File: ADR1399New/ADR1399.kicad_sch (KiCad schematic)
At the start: 95 parts, among them J1 GNDF_SPARE, J10 Conn_01x01_Male, J11 Conn_01x01, J2 10V, J3 PT100, J4 Guards, J5 7V, J6 Conn_01x02_Male, J7 Conn_01x02_Male, J8 Conn_01x02_Male, J9 Conn_01x02_Male, Q1 BC817, U1 OPA2182xD, U2 OPA2209xD, U3 OPA2182xD, U4 LM399, U5 LM7905_TO220, U6 LM7815_TO220, U7 LM7805_TO220, U8 OPA2182xD

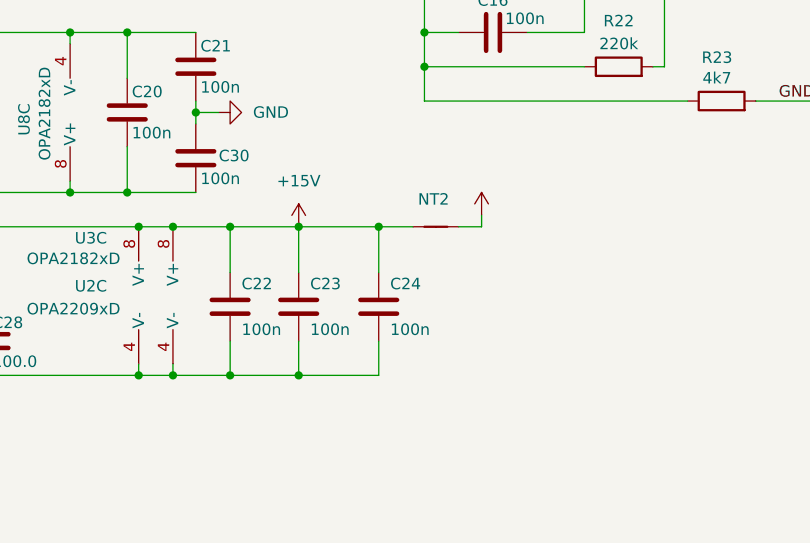
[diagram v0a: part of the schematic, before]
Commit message: Update KiCad project and backup files- just before format R9 7900x SSD
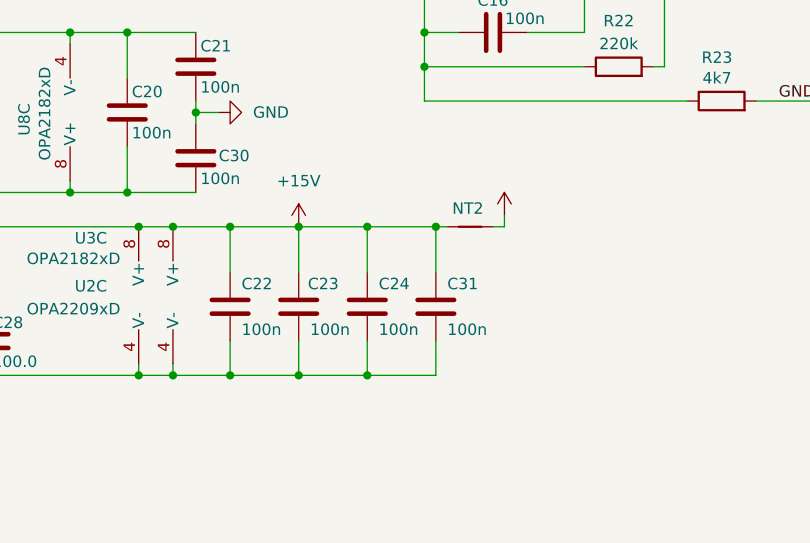
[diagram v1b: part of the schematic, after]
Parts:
- added C31: 100n, Capacitor_SMD:C_0805_2012Metric_Pad1.18x1.45mm_HandSolder, symbol Device:C
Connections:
- net +15V: now also C31.1
- net GND: now also C31.2
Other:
- moved on the sheet: C24, NT2
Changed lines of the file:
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@@
 	)
 	(junction
+		(at 134.62 163.83)
+		(diameter 0)
+		(color 0 0 0 0)
+	)
+	(junction
 		(at 31.75 63.5)
 		(diameter 0)
@@
 	)
 	(junction
+		(at 142.24 163.83)
+		(diameter 0)
+		(color 0 0 0 0)
+	)
+	(junction
 		(at 129.54 57.15)
 		(diameter 0)
@@
 	)
 	(junction
-		(at 135.89 163.83)
-		(diameter 0)
-		(color 0 0 0 0)
-	)
-	(junction
 		(at 63.5 180.34)
 		(diameter 0)
@@
 	)
 	(junction
+		(at 134.62 180.34)
+		(diameter 0)
+		(color 0 0 0 0)
+	)
+	(junction
 		(at 63.5 154.94)
 		(diameter 0)
@@
 	(wire
 		(pts
-			(xy 147.32 162.56) (xy 147.32 163.83)
+			(xy 149.86 162.56) (xy 149.86 163.83)
 		)
 		(stroke
@@
 	(wire
 		(pts
-			(xy 127 180.34) (xy 135.89 180.34)
+			(xy 127 180.34) (xy 134.62 180.34)
 		)
 		(stroke
@@
 	(wire
 		(pts
+			(xy 134.62 180.34) (xy 142.24 180.34)
+		)
+		(stroke
+			(width 0)
+			(type default)
+		)
+	)
+	(wire
+		(pts
 			(xy 132.08 97.79) (xy 137.16 97.79)
 		)
@@
 	(wire
 		(pts
-			(xy 127 163.83) (xy 135.89 163.83)
+			(xy 127 163.83) (xy 134.62 163.83)
 		)
 		(stroke
@@
 	(wire
 		(pts
+			(xy 142.24 163.83) (xy 143.51 163.83)
+		)
+		(stroke
+			(width 0)
+			(type default)
+		)
+	)
+	(wire
+		(pts
 			(xy 68.58 57.15) (xy 68.58 58.42)
 		)
@@
 	(wire
 		(pts
-			(xy 135.89 163.83) (xy 139.7 163.83)
-		)
-		(stroke
-			(width 0)
-			(type default)
-		)
-	)
-	(wire
-		(pts
 			(xy 115.57 149.86) (xy 115.57 151.13)
 		)
@@
 	(wire
 		(pts
+			(xy 142.24 163.83) (xy 142.24 168.91)
+		)
+		(stroke
+			(width 0)
+			(type default)
+		)
+	)
+	(wire
+		(pts
 			(xy 123.19 105.41) (xy 123.19 110.49)
 		)
@@
 	(wire
 		(pts
-			(xy 135.89 176.53) (xy 135.89 180.34)
+			(xy 134.62 176.53) (xy 134.62 180.34)
 		)
 		(stroke
@@
 	(wire
 		(pts
-			(xy 144.78 163.83) (xy 147.32 163.83)
+			(xy 148.59 163.83) (xy 149.86 163.83)
 		)
 		(stroke
@@
 	(wire
 		(pts
-			(xy 135.89 163.83) (xy 135.89 168.91)
+			(xy 134.62 163.83) (xy 134.62 168.91)
 		)
 		(stroke
@@
 	(wire
 		(pts
+			(xy 142.24 176.53) (xy 142.24 180.34)
+		)
+		(stroke
+			(width 0)
+			(type default)
+		)
+	)
+	(wire
+		(pts
 			(xy 185.42 34.29) (xy 189.23 34.29)
 		)
@@
 	(wire
 		(pts
+			(xy 134.62 163.83) (xy 142.24 163.83)
+		)
+		(stroke
+			(width 0)
+			(type default)
+		)
+	)
+	(wire
+		(pts
 			(xy 127 78.74) (xy 127 80.01)
 		)
@@
 	(symbol
 		(lib_id "Device:NetTie_2")
-		(at 142.24 163.83 0)
+		(at 146.05 163.83 0)
 		(unit 1)
 		(exclude_from_sim no)
@@
 		(dnp no)
 		(property "Reference" "NT2"
-			(at 141.986 160.782 0)
+			(at 145.796 161.798 0)
 			(effects
 				(font
@@
 		)
 		(property "Value" "NetTie_2"
-			(at 142.24 161.29 0)
+			(at 146.05 161.29 0)
 			(effects
 				(font
@@
 		)
 		(property "Footprint" "NetTie:NetTie-2_SMD_Pad2.0mm"
-			(at 142.24 163.83 0)
+			(at 146.05 163.83 0)
 			(effects
 				(font
@@
 		)
 		(property "Datasheet" "~"
-			(at 142.24 163.83 0)
+			(at 146.05 163.83 0)
 			(effects
 				(font
@@
 		)
 		(property "Description" "Net tie, 2 pins"
-			(at 142.24 163.83 0)
+			(at 146.05 163.83 0)
 			(effects
 				(font
@@
 	(symbol
 		(lib_id "power:+24V")
-		(at 147.32 162.56 0)
+		(at 149.86 162.56 0)
 		(unit 1)
 		(exclude_from_sim no)
@@
 		(fields_autoplaced yes)
 		(property "Reference" "#PWR022"
-			(at 147.32 166.37 0)
+			(at 149.86 166.37 0)
 			(effects
 				(font
@@
 		)
 		(property "Value" "+24V"
-			(at 147.32 157.48 0)
+			(at 149.86 157.48 0)
 			(effects
 				(font
@@
 		)
 		(property "Footprint" ""
-			(at 147.32 162.56 0)
+			(at 149.86 162.56 0)
 			(effects
 				(font
@@
 		)
 		(property "Datasheet" ""
-			(at 147.32 162.56 0)
+			(at 149.86 162.56 0)
 			(effects
 				(font
@@
 		)
 		(property "Description" "Power symbol creates a global label with name \"+24V\""
-			(at 147.32 162.56 0)
+			(at 149.86 162.56 0)
 			(effects
 				(font
@@
 	)
 	(symbol
+		(lib_id "Device:C")
+		(at 142.24 172.72 0)
+		(unit 1)
+		(exclude_from_sim no)
+		(in_bom yes)
+		(on_board yes)
+		(dnp no)
+		(property "Reference" "C31"
+			(at 143.51 170.18 0)
+			(effects
+				(font
+					(size 1.27 1.27)
+				)
+				(justify left)
+			)
+		)
+		(property "Value" "100n"
+			(at 143.51 175.26 0)
+			(effects
+				(font
+					(size 1.27 1.27)
+				)
+				(justify left)
+			)
+		)
+		(property "Footprint" "Capacitor_SMD:C_0805_2012Metric_Pad1.18x1.45mm_HandSolder"
+			(at 143.2052 176.53 0)
+			(effects
+				(font
+					(size 1.27 1.27)
+				)
+				(hide yes)
+			)
+		)
+		(property "Datasheet" "~"
+			(at 142.24 172.72 0)
+			(effects
+				(font
+					(size 1.27 1.27)
+				)
+				(hide yes)
+			)
+		)
+		(property "Description" "Unpolarized capacitor"
+			(at 142.24 172.72 0)
+			(effects
+				(font
+					(size 1.27 1.27)
+				)
+				(hide yes)
+			)
+		)
+		(pin "1"
+		)
+		(pin "2"
+		)
+		(instances
+			(project "ADR1399"
+				(path "/e63e39d7-6ac0-4ffd-8aa3-1841a4541b55"
+					(reference "C31")
+					(unit 1)
+				)
+			)
+		)
+	)
+	(symbol
 		(lib_id "Device:R")
 		(at 39.37 187.96 0)
@@
 		(dnp no)
 		(property "Reference" "C23"
-			(at 128.27 170.18 0)
+			(at 128.016 170.18 0)
 			(effects
 				(font
@@
 	(symbol
 		(lib_id "Device:C")
-		(at 135.89 172.72 0)
+		(at 134.62 172.72 0)
 		(unit 1)
 		(exclude_from_sim no)
@@
 		(dnp no)
 		(property "Reference" "C24"
-			(at 137.16 170.18 0)
+			(at 135.89 170.18 0)
 			(effects
 				(font
@@
 		)
 		(property "Value" "100n"
-			(at 137.16 175.26 0)
+			(at 135.89 175.26 0)
 			(effects
 				(font
@@
 		)
 		(property "Footprint" "Capacitor_SMD:C_0805_2012Metric_Pad1.18x1.45mm_HandSolder"
-			(at 136.8552 176.53 0)
+			(at 135.5852 176.53 0)
 			(effects
 				(font
@@
 		)
 		(property "Datasheet" "~"
-			(at 135.89 172.72 0)
+			(at 134.62 172.72 0)
 			(effects
 				(font
@@
 		)
 		(property "Description" "Unpolarized capacitor"
-			(at 135.89 172.72 0)
+			(at 134.62 172.72 0)
 			(effects
 				(font
